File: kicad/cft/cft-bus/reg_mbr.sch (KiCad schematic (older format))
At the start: 22 parts, among them U14 74AHC1G125, U28 74HC670, U29 74HC670, U30 74HC541, U31 74HC139, U33 74HC670, U34 74HC670, U35 74LVC1G74, U36 74AHC1G125, U39 74HC139, U40 74LVC1G74

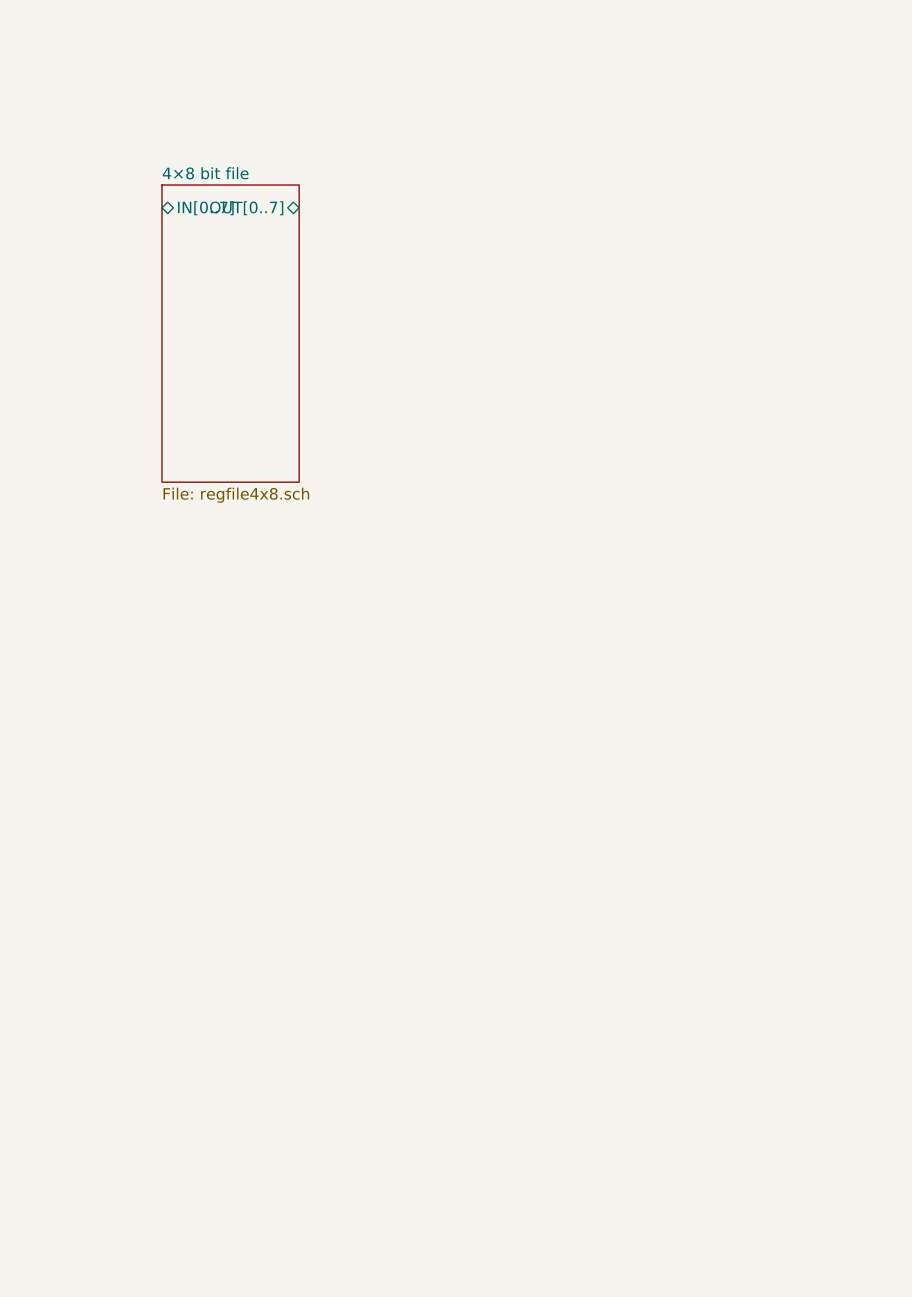
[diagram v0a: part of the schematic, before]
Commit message: A little work on the BUS card
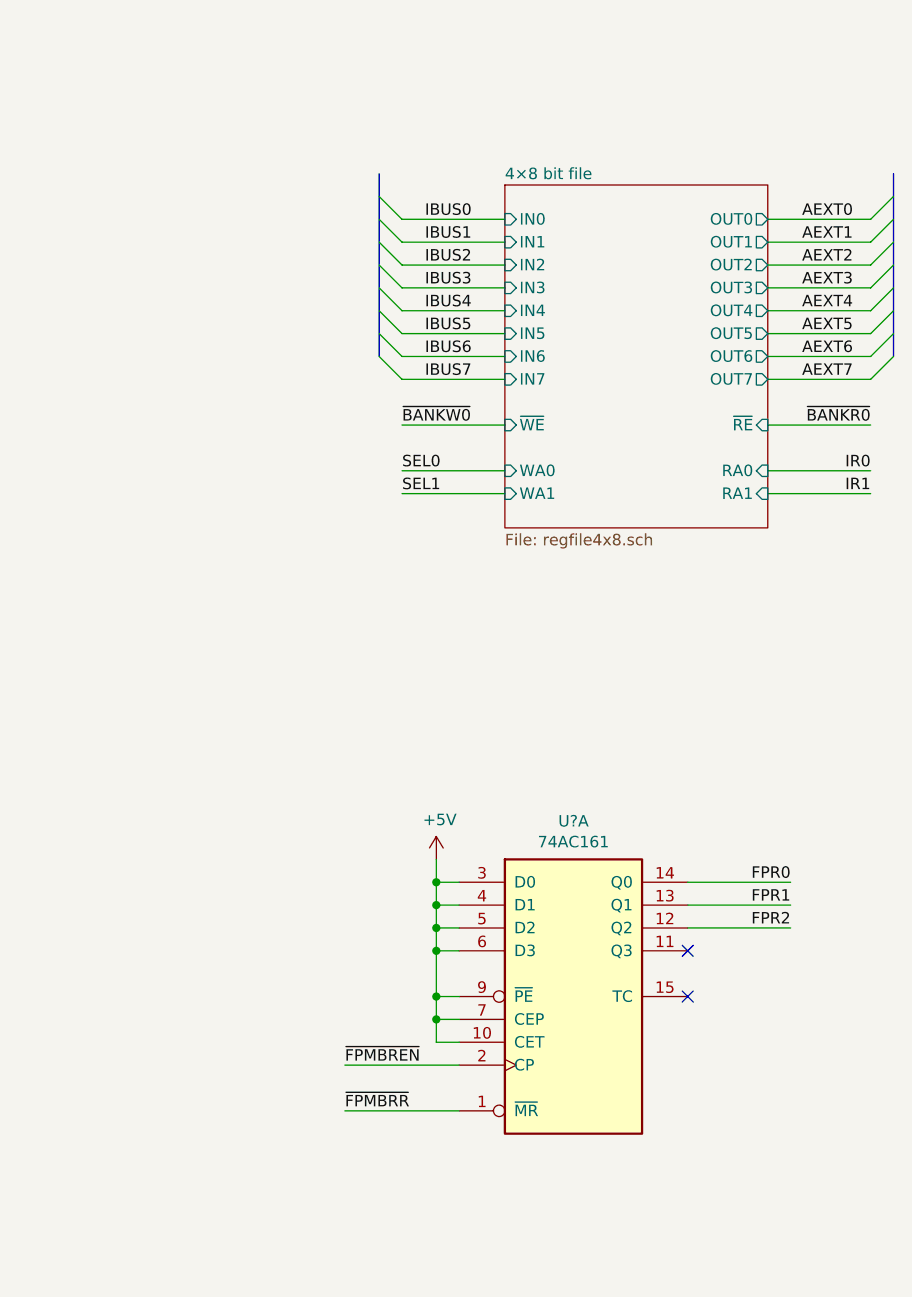
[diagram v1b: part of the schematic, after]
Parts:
- added U?: 74AC161, symbol alexios:74AC161
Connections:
- net +5V: now also U?.10 (CET), U?.3 (D0), U?.4 (D1), U?.5 (D2), U?.6 (D3), U?.7 (CEP), U?.9 (~PE)
- new net FPR0: U?.14 (Q0)
- new net FPR1: U?.13 (Q1)
- new net FPR2: U?.12 (Q2)
- new net ~FPMBREN: U?.2 (CP)
- new net ~FPMBRR: U?.1 (~MR)
- no-connect marks 4 -> 6
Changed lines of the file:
@@
 Rev ""
 Comp ""
-Comment1 "CTL"
+Comment1 "BUS"
 Comment2 ""
 Comment3 ""
@@
 Text Notes 8250 2950 0    50   ~ 10
 Note
+$Sheet
+S 13400 1400 1150 1500
+U 5E647D2E
+F0 "4×8 bit file" 50
+F1 "regfile4x8.sch" 50
+F2 "WA0" I L 13400 2650 50
+F3 "WA1" I L 13400 2750 50
+F4 "RA0" I R 14550 2650 50
+F5 "RA1" I R 14550 2750 50
+F6 "~RE" I R 14550 2450 50
+F7 "~WE" I L 13400 2450 50
+F8 "IN0" I L 13400 1550 50
+F9 "IN1" I L 13400 1650 50
+F10 "IN2" I L 13400 1750 50
+F11 "IN3" I L 13400 1850 50
+F12 "IN4" I L 13400 1950 50
+F13 "IN5" I L 13400 2050 50
+F14 "IN6" I L 13400 2150 50
+F15 "IN7" I L 13400 2250 50
+F16 "OUT0" O R 14550 1550 50
+F17 "OUT1" O R 14550 1650 50
+F18 "OUT2" O R 14550 1750 50
+F19 "OUT3" O R 14550 1850 50
+F20 "OUT4" O R 14550 1950 50
+F21 "OUT5" O R 14550 2050 50
+F22 "OUT6" O R 14550 2150 50
+F23 "OUT7" O R 14550 2250 50
+$EndSheet
+Text Label 14700 1850 0    50   ~ 0
+AEXT3
+Text Label 14700 1750 0    50   ~ 0
+AEXT2
+Text Label 14700 1650 0    50   ~ 0
+AEXT1
+Text Label 14700 1550 0    50   ~ 0
+AEXT0
+Wire Wire Line
+	14550 1850 15000 1850
+Wire Wire Line
+	14550 1750 15000 1750
+Wire Wire Line
+	14550 1650 15000 1650
+Wire Wire Line
+	14550 1550 15000 1550
+Text Label 14700 1950 0    50   ~ 0
+AEXT4
+Text Label 14700 2050 0    50   ~ 0
+AEXT5
+Text Label 14700 2150 0    50   ~ 0
+AEXT6
+Text Label 14700 2250 0    50   ~ 0
+AEXT7
+Wire Wire Line
+	14550 1950 15000 1950
+Wire Wire Line
+	14550 2250 15000 2250
+Wire Wire Line
+	14550 2150 15000 2150
+Wire Wire Line
+	14550 2050 15000 2050
+Wire Wire Line
+	13400 1850 12950 1850
+Wire Wire Line
+	13400 1750 12950 1750
+Wire Wire Line
+	13400 1650 12950 1650
+Wire Wire Line
+	13400 1550 12950 1550
+Entry Wire Line
+	12950 1950 12850 1850
+Entry Wire Line
+	12950 2050 12850 1950
+Entry Wire Line
+	12950 2150 12850 2050
+Entry Wire Line
+	12950 2250 12850 2150
+Entry Wire Line
+	12950 1550 12850 1450
+Entry Wire Line
+	12950 1650 12850 1550
+Entry Wire Line
+	12950 1750 12850 1650
+Entry Wire Line
+	12950 1850 12850 1750
+Wire Wire Line
+	13400 1950 12950 1950
+Wire Wire Line
+	13400 2250 12950 2250
+Wire Wire Line
+	13400 2150 12950 2150
+Wire Wire Line
+	13400 2050 12950 2050
+Text Label 13050 1550 0    50   ~ 0
+IBUS0
+Text Label 13050 1650 0    50   ~ 0
+IBUS1
+Text Label 13050 1750 0    50   ~ 0
+IBUS2
+Text Label 13050 1850 0    50   ~ 0
+IBUS3
+Text Label 13050 1950 0    50   ~ 0
+IBUS4
+Text Label 13050 2050 0    50   ~ 0
+IBUS5
+Text Label 13050 2150 0    50   ~ 0
+IBUS6
+Text Label 13050 2250 0    50   ~ 0
+IBUS7
+Wire Wire Line
+	13400 2450 12950 2450
+Wire Wire Line
+	13400 2650 12950 2650
+Wire Wire Line
+	13400 2750 12950 2750
+Text Label 12950 2650 0    50   ~ 0
+SEL0
+Text Label 12950 2750 0    50   ~ 0
+SEL1
+Text Label 12950 2450 0    50   ~ 0
+~BANKW0
+Entry Wire Line
+	15000 1950 15100 1850
+Entry Wire Line
+	15000 2050 15100 1950
+Entry Wire Line
+	15000 2150 15100 2050
+Entry Wire Line
+	15000 2250 15100 2150
+Entry Wire Line
+	15000 1550 15100 1450
+Entry Wire Line
+	15000 1650 15100 1550
+Entry Wire Line
+	15000 1750 15100 1650
+Entry Wire Line
+	15000 1850 15100 1750
+Wire Wire Line
+	14550 2450 15000 2450
+Wire Wire Line
+	14550 2650 15000 2650
+Wire Wire Line
+	14550 2750 15000 2750
+Text Label 15000 2450 2    50   ~ 0
+~BANKR0
+Text Label 15000 2650 2    50   ~ 0
+IR0
+Text Label 15000 2750 2    50   ~ 0
+IR1
+$Comp
+L alexios:74AC161 U?
+U 1 1 5DF5E120
+P 13700 4950
+F 0 "U?" H 13700 5717 50  0000 C CNN
+F 1 "74AC161" H 13700 5626 50  0000 C CNN
+F 2 "" H 14000 5200 50  0001 C CNN
+F 3 "https://assets.nexperia.com/documents/data-sheet/74HC161.pdf" H 14000 5200 50  0001 C CNN
+	1    13700 4950
+	1    0    0    -1
+$EndComp
+Wire Wire Line
+	14200 4450 14650 4450
+Wire Wire Line
+	14200 4550 14650 4550
+Wire Wire Line
+	14200 4650 14650 4650
+Text Label 14650 4450 2    50   ~ 0
+FPR0
+Text Label 14650 4550 2    50   ~ 0
+FPR1
+Text Label 14650 4650 2    50   ~ 0
+FPR2
+NoConn ~ 14200 4750
+NoConn ~ 14200 4950
+Wire Wire Line
+	13200 5050 13100 5050
+$Comp
+L power:+5V #PWR?
+U 1 1 5DFAEFFD
+P 13100 4350
+F 0 "#PWR?" H 13100 4200 50  0001 C CNN
+F 1 "+5V" H 13115 4523 50  0000 C CNN
+F 2 "" H 13100 4350 50  0001 C CNN
+F 3 "" H 13100 4350 50  0001 C CNN
+	1    13100 4350
+	1    0    0    -1
+$EndComp
+Wire Wire Line
+	13200 5150 13100 5150
+Wire Wire Line
+	13200 5250 12700 5250
+Text Label 12700 5250 0    50   ~ 0
+~FPMBREN
+Wire Wire Line
+	13200 5450 12700 5450
+Text Label 12700 5450 0    50   ~ 0
+~FPMBRR
+Wire Wire Line
+	13100 5150 13100 5050
+Connection ~ 13100 5050
+Wire Wire Line
+	13100 5050 13100 4950
+Wire Wire Line
+	13200 4450 13100 4450
+Connection ~ 13100 4450
+Wire Wire Line
+	13100 4450 13100 4350
+Wire Wire Line
+	13200 4550 13100 4550
+Connection ~ 13100 4550
+Wire Wire Line
+	13100 4550 13100 4450
+Wire Wire Line
+	13200 4650 13100 4650
+Connection ~ 13100 4650
+Wire Wire Line
+	13100 4650 13100 4550
+Wire Wire Line
+	13200 4750 13100 4750
+Connection ~ 13100 4750
+Wire Wire Line
+	13100 4750 13100 4650
+Wire Wire Line
+	13200 4950 13100 4950
+Connection ~ 13100 4950
+Wire Wire Line
+	13100 4950 13100 4750
+Wire Bus Line
+	12850 1350 12850 2150
+Wire Bus Line
+	15100 1350 15100 2150
 Wire Bus Line
 	3700 800  3700 3300
@@
 Wire Bus Line
 	7650 1600 7650 4400
-$Sheet
-S 11900 1400 600  1300
-U 5E647D2E
-F0 "4×8 bit file" 50
-F1 "regfile4x8.sch" 50
-F2 "OUT[0..7]" T R 12500 1500 50
-F3 "IN[0..7]" T L 11900 1500 50
-$EndSheet
 $EndSCHEMATC
